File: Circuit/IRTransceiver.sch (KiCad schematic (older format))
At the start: 4 parts

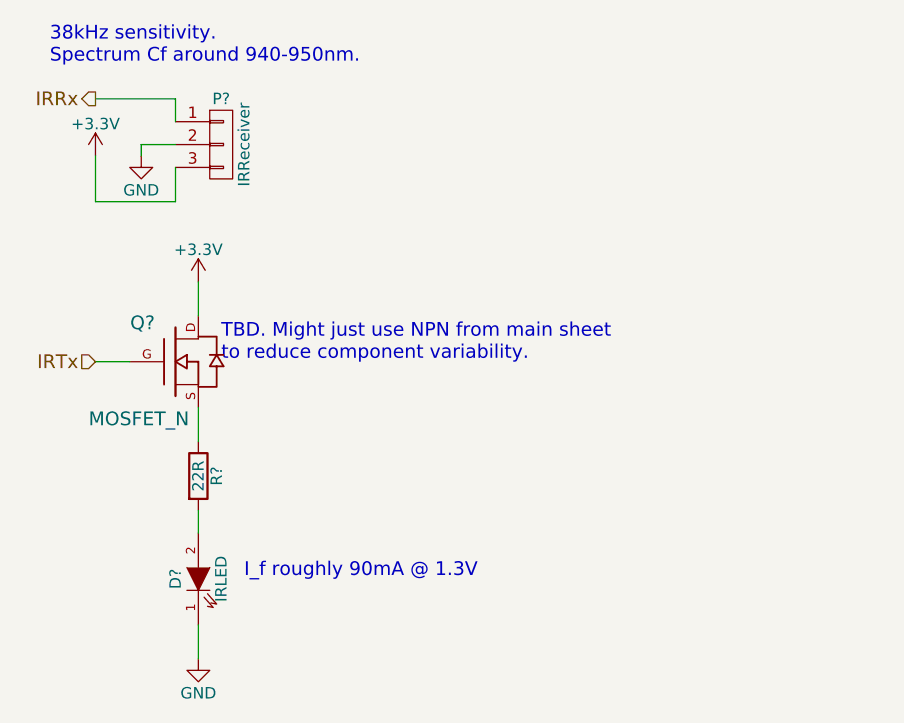
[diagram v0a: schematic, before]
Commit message: Messing with John's layout. You're welcome.
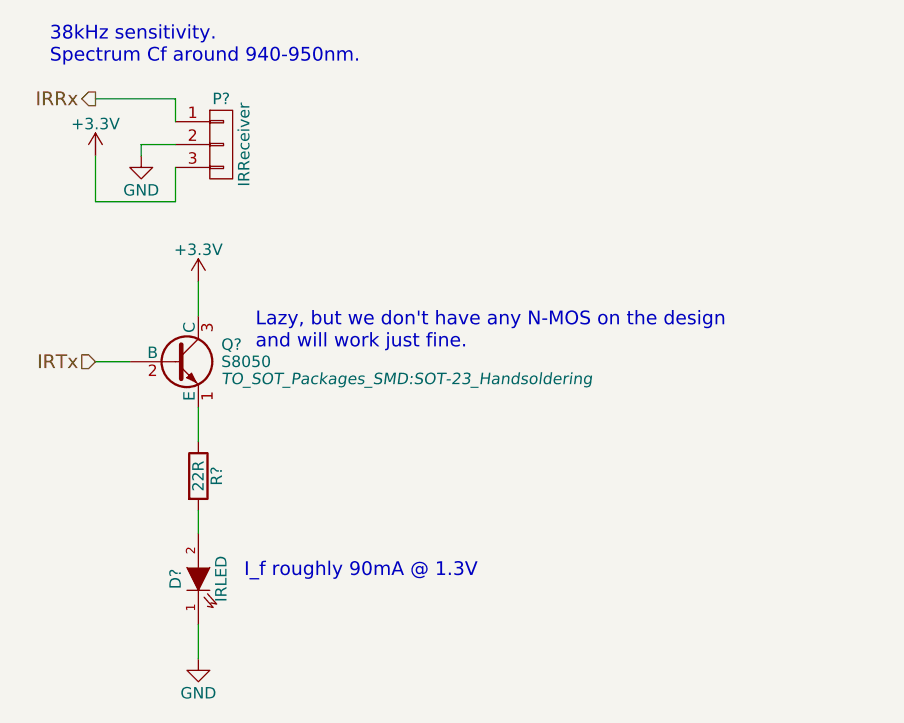
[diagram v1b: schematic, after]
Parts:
- removed Q?: MOSFET_N, symbol MOSFET_N
- added Q?: S8050, TO_SOT_Packages_SMD:SOT-23_Handsoldering, symbol S8050
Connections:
- net +3V3: now also Q?.3 (C)
- net IRTx: now also Q?.2 (B)
- net at R?.1: now also Q?.1 (E)
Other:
- note added: "Lazy, but we don't have any N-MOS on the design\nand will work just fine."
- note removed: "TBD. Might just use NPN from main sheet\nto reduce component variability."
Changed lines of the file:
@@
 Wire Wire Line
 	4500 4300 4500 4400
-$Comp
-L MOSFET_N Q?
-U 1 1 581D6A1D
-P 4400 3650
-F 0 "Q?" H 4310 3820 60  0000 R CNN
-F 1 "MOSFET_N" H 4460 3400 60  0000 R CNN
-F 2 "" H 4400 3650 60  0000 C CNN
-F 3 "" H 4400 3650 60  0000 C CNN
-	1    4400 3650
-	1    0    0    -1
-$EndComp
 Wire Wire Line
 	4500 3850 4500 4000
@@
 Text Notes 4700 4600 0    60   ~ 0
 I_f roughly 90mA @ 1.3V
-Text Notes 4600 3650 0    60   ~ 0
-TBD. Might just use NPN from main sheet\nto reduce component variability.
+Text Notes 4750 3600 0    60   ~ 0
+Lazy, but we don't have any N-MOS on the design\nand will work just fine.
+$Comp
+L S8050 Q?
+U 1 1 581E1075
+P 4400 3650
+F 0 "Q?" H 4600 3725 50  0000 L CNN
+F 1 "S8050" H 4600 3650 50  0000 L CNN
+F 2 "TO_SOT_Packages_SMD:SOT-23_Handsoldering" H 4600 3575 50  0000 L CIN
+F 3 "" H 4400 3650 50  0000 L CNN
+	1    4400 3650
+	1    0    0    -1
+$EndComp
 $EndSCHEMATC
